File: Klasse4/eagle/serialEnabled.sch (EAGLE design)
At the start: 3 parts

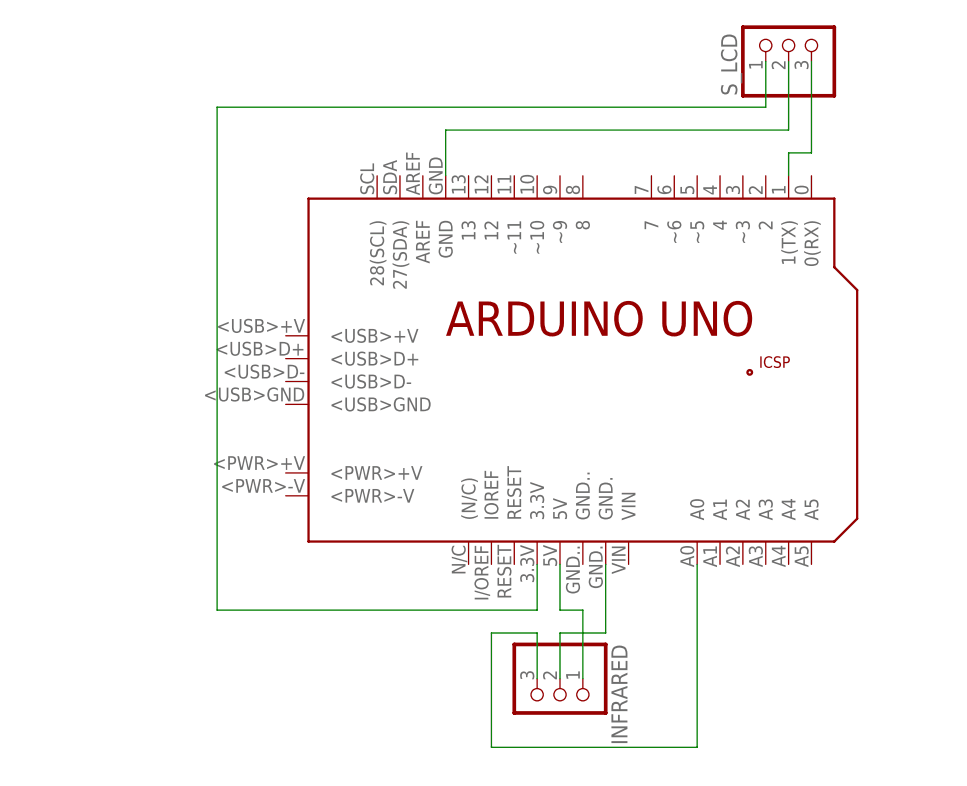
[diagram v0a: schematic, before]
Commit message: update
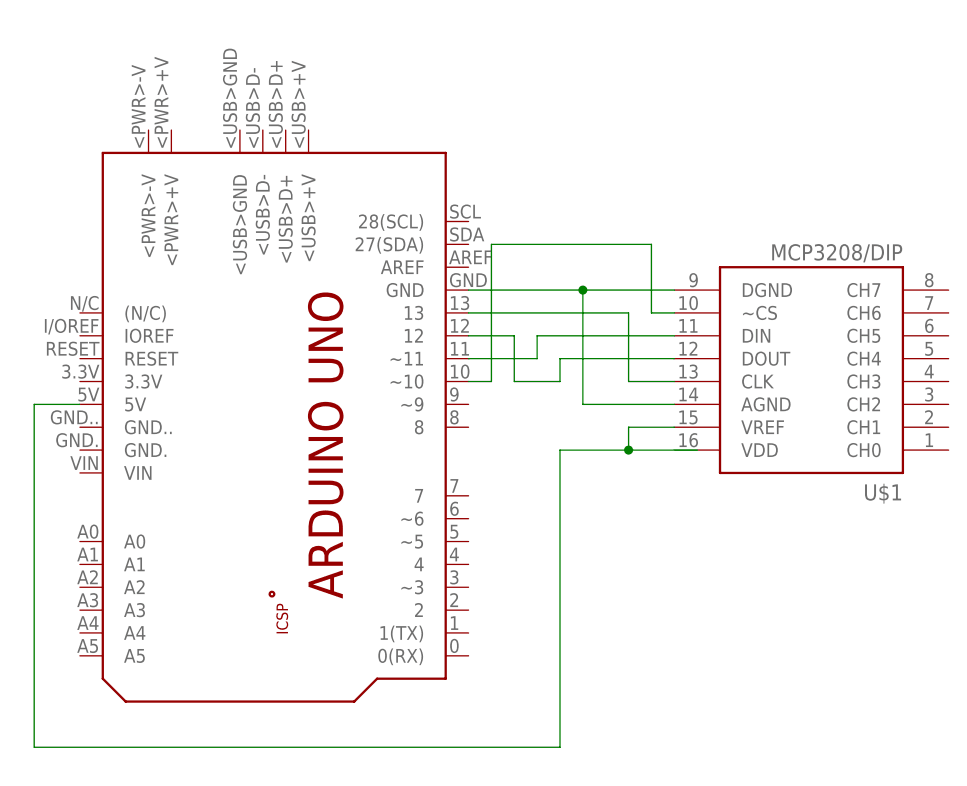
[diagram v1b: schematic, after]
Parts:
- removed INFRARED, S_LCD: (no value), pinhead:PINHD-1X3
- added U$1: MCP3208/DIP, mcp3208:MCP3208/DIP
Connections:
- net N$1: now also PCB1.GND, U$1.AGND, U$1.DGND; no longer INFRARED.1, PCB1.5V
- net N$2: now also PCB1.~11, U$1.DIN; no longer INFRARED.2, PCB1.GND.
- net N$3: now also PCB1.5V, U$1.VREF; no longer INFRARED.3, PCB1.A0
- net N$4: now also PCB1.13, U$1.CLK; no longer PCB1.1(TX), S_LCD.3
- net N$5: now also PCB1.12, U$1.DOUT; no longer PCB1.GND, S_LCD.2
- net N$6: now also PCB1.~10, U$1.~CS; no longer PCB1.3.3V, S_LCD.1
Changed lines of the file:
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@@
 <layer number="106" name="bPlate" color="7" fill="1" visible="yes" active="yes"/>
 <layer number="107" name="Crop" color="7" fill="1" visible="yes" active="yes"/>
+<layer number="108" name="fp8" color="7" fill="1" visible="no" active="yes"/>
+<layer number="109" name="fp9" color="7" fill="1" visible="no" active="yes"/>
+<layer number="110" name="fp0" color="7" fill="1" visible="no" active="yes"/>
+<layer number="111" name="LPC17xx" color="7" fill="1" visible="yes" active="yes"/>
 <layer number="116" name="Patch_BOT" color="9" fill="4" visible="yes" active="yes"/>
 <layer number="121" name="_tsilk" color="7" fill="1" visible="yes" active="yes"/>
 <layer number="122" name="_bsilk" color="7" fill="1" visible="yes" active="yes"/>
+<layer number="123" name="tTestmark" color="7" fill="1" visible="no" active="yes"/>
+<layer number="124" name="bTestmark" color="7" fill="1" visible="no" active="yes"/>
 <layer number="125" name="_tNames" color="7" fill="1" visible="yes" active="yes"/>
+<layer number="131" name="tAdjust" color="7" fill="1" visible="no" active="yes"/>
+<layer number="132" name="bAdjust" color="7" fill="1" visible="no" active="yes"/>
 <layer number="144" name="Drill_legend" color="7" fill="1" visible="yes" active="yes"/>
 <layer number="151" name="HeatSink" color="7" fill="1" visible="yes" active="yes"/>
+<layer number="199" name="Contour" color="7" fill="1" visible="yes" active="yes"/>
 <layer number="200" name="200bmp" color="1" fill="10" visible="yes" active="yes"/>
 <layer number="201" name="201bmp" color="2" fill="10" visible="yes" active="yes"/>
@@
 <parts>
 <part name="PCB1" library="E14_Arduino" deviceset="ARDUINO_UNO" device=""/>
-<part name="INFRARED" library="pinhead" deviceset="PINHD-1X3" device=""/>
-<part name="S_LCD" library="pinhead" deviceset="PINHD-1X3" device=""/>
+<part name="U$1" library="mcp3208" deviceset="MCP3208/DIP" device=""/>
 </parts>
 <sheets>
@@
 </plain>
 <instances>
-<instance part="PCB1" gate="G$1" x="2.54" y="30.48"/>
-<instance part="INFRARED" gate="A" x="0" y="-7.62" rot="R270"/>
-<instance part="S_LCD" gate="A" x="25.4" y="66.04" rot="R90"/>
+<instance part="PCB1" gate="G$1" x="-30.48" y="22.86" rot="R270"/>
+<instance part="U$1" gate="G$1" x="27.94" y="30.48" rot="R180"/>
 </instances>
 <busses>
@@
 <net name="N$1" class="0">
 <segment>
+<pinref part="PCB1" gate="G$1" pin="GND"/>
+<pinref part="U$1" gate="G$1" pin="DGND"/>
+<wire x1="-10.16" y1="38.1" x2="2.54" y2="38.1" width="0.1524" layer="91"/>
+<pinref part="U$1" gate="G$1" pin="AGND"/>
+<wire x1="2.54" y1="38.1" x2="12.7" y2="38.1" width="0.1524" layer="91"/>
+<wire x1="12.7" y1="25.4" x2="2.54" y2="25.4" width="0.1524" layer="91"/>
+<wire x1="2.54" y1="25.4" x2="2.54" y2="38.1" width="0.1524" layer="91"/>
+<junction x="2.54" y="38.1"/>
+</segment>
+</net>
+<net name="N$3" class="0">
+<segment>
 <pinref part="PCB1" gate="G$1" pin="5V"/>
-<wire x1="0" y1="7.62" x2="0" y2="2.54" width="0.1524" layer="91"/>
-<wire x1="0" y1="2.54" x2="2.54" y2="2.54" width="0.1524" layer="91"/>
-<pinref part="INFRARED" gate="A" pin="1"/>
-<wire x1="2.54" y1="2.54" x2="2.54" y2="-5.08" width="0.1524" layer="91"/>
+<wire x1="-53.34" y1="25.4" x2="-58.42" y2="25.4" width="0.1524" layer="91"/>
+<wire x1="-58.42" y1="25.4" x2="-58.42" y2="-12.7" width="0.1524" layer="91"/>
+<wire x1="-58.42" y1="-12.7" x2="0" y2="-12.7" width="0.1524" layer="91"/>
+<wire x1="0" y1="-12.7" x2="0" y2="20.32" width="0.1524" layer="91"/>
+<wire x1="0" y1="20.32" x2="7.62" y2="20.32" width="0.1524" layer="91"/>
+<pinref part="U$1" gate="G$1" pin="VREF"/>
+<wire x1="7.62" y1="20.32" x2="15.24" y2="20.32" width="0.1524" layer="91"/>
+<wire x1="12.7" y1="22.86" x2="7.62" y2="22.86" width="0.1524" layer="91"/>
+<wire x1="7.62" y1="22.86" x2="7.62" y2="20.32" width="0.1524" layer="91"/>
+<junction x="7.62" y="20.32"/>
 </segment>
 </net>
 <net name="N$2" class="0">
 <segment>
-<pinref part="PCB1" gate="G$1" pin="GND."/>
-<wire x1="5.08" y1="7.62" x2="5.08" y2="0" width="0.1524" layer="91"/>
-<wire x1="5.08" y1="0" x2="0" y2="0" width="0.1524" layer="91"/>
-<pinref part="INFRARED" gate="A" pin="2"/>
-<wire x1="0" y1="0" x2="0" y2="-5.08" width="0.1524" layer="91"/>
-</segment>
-</net>
-<net name="N$3" class="0">
-<segment>
-<pinref part="INFRARED" gate="A" pin="3"/>
-<wire x1="-2.54" y1="-5.08" x2="-2.54" y2="0" width="0.1524" layer="91"/>
-<wire x1="-2.54" y1="0" x2="-7.62" y2="0" width="0.1524" layer="91"/>
-<wire x1="-7.62" y1="0" x2="-7.62" y2="-12.7" width="0.1524" layer="91"/>
-<pinref part="PCB1" gate="G$1" pin="A0"/>
-<wire x1="-7.62" y1="-12.7" x2="15.24" y2="-12.7" width="0.1524" layer="91"/>
-<wire x1="15.24" y1="-12.7" x2="15.24" y2="7.62" width="0.1524" layer="91"/>
+<pinref part="PCB1" gate="G$1" pin="~11"/>
+<wire x1="-10.16" y1="30.48" x2="-2.54" y2="30.48" width="0.1524" layer="91"/>
+<wire x1="-2.54" y1="30.48" x2="-2.54" y2="33.02" width="0.1524" layer="91"/>
+<pinref part="U$1" gate="G$1" pin="DIN"/>
+<wire x1="12.7" y1="33.02" x2="-2.54" y2="33.02" width="0.1524" layer="91"/>
 </segment>
 </net>
 <net name="N$4" class="0">
 <segment>
-<pinref part="S_LCD" gate="A" pin="3"/>
-<wire x1="27.94" y1="63.5" x2="27.94" y2="53.34" width="0.1524" layer="91"/>
-<wire x1="27.94" y1="53.34" x2="25.4" y2="53.34" width="0.1524" layer="91"/>
-<pinref part="PCB1" gate="G$1" pin="1(TX)"/>
-<wire x1="25.4" y1="53.34" x2="25.4" y2="50.8" width="0.1524" layer="91"/>
+<pinref part="PCB1" gate="G$1" pin="13"/>
+<wire x1="-10.16" y1="35.56" x2="7.62" y2="35.56" width="0.1524" layer="91"/>
+<wire x1="7.62" y1="35.56" x2="7.62" y2="27.94" width="0.1524" layer="91"/>
+<pinref part="U$1" gate="G$1" pin="CLK"/>
+<wire x1="7.62" y1="27.94" x2="12.7" y2="27.94" width="0.1524" layer="91"/>
 </segment>
 </net>
 <net name="N$5" class="0">
 <segment>
-<pinref part="S_LCD" gate="A" pin="2"/>
-<wire x1="25.4" y1="63.5" x2="25.4" y2="55.88" width="0.1524" layer="91"/>
-<wire x1="25.4" y1="55.88" x2="-12.7" y2="55.88" width="0.1524" layer="91"/>
-<pinref part="PCB1" gate="G$1" pin="GND"/>
-<wire x1="-12.7" y1="55.88" x2="-12.7" y2="50.8" width="0.1524" layer="91"/>
+<pinref part="PCB1" gate="G$1" pin="12"/>
+<wire x1="-10.16" y1="33.02" x2="-5.08" y2="33.02" width="0.1524" layer="91"/>
+<wire x1="-5.08" y1="33.02" x2="-5.08" y2="27.94" width="0.1524" layer="91"/>
+<wire x1="-5.08" y1="27.94" x2="0" y2="27.94" width="0.1524" layer="91"/>
+<wire x1="0" y1="27.94" x2="0" y2="30.48" width="0.1524" layer="91"/>
+<pinref part="U$1" gate="G$1" pin="DOUT"/>
+<wire x1="0" y1="30.48" x2="12.7" y2="30.48" width="0.1524" layer="91"/>
 </segment>
 </net>
 <net name="N$6" class="0">
 <segment>
-<pinref part="S_LCD" gate="A" pin="1"/>
-<wire x1="22.86" y1="63.5" x2="22.86" y2="58.42" width="0.1524" layer="91"/>
-<wire x1="22.86" y1="58.42" x2="-38.1" y2="58.42" width="0.1524" layer="91"/>
-<wire x1="-38.1" y1="58.42" x2="-38.1" y2="2.54" width="0.1524" layer="91"/>
-<pinref part="PCB1" gate="G$1" pin="3.3V"/>
-<wire x1="-38.1" y1="2.54" x2="-2.54" y2="2.54" width="0.1524" layer="91"/>
-<wire x1="-2.54" y1="2.54" x2="-2.54" y2="7.62" width="0.1524" layer="91"/>
+<pinref part="PCB1" gate="G$1" pin="~10"/>
+<wire x1="-10.16" y1="27.94" x2="-7.62" y2="27.94" width="0.1524" layer="91"/>
+<wire x1="-7.62" y1="27.94" x2="-7.62" y2="43.18" width="0.1524" layer="91"/>
+<wire x1="-7.62" y1="43.18" x2="10.16" y2="43.18" width="0.1524" layer="91"/>
+<wire x1="10.16" y1="43.18" x2="10.16" y2="35.56" width="0.1524" layer="91"/>
+<pinref part="U$1" gate="G$1" pin="~CS"/>
+<wire x1="10.16" y1="35.56" x2="12.7" y2="35.56" width="0.1524" layer="91"/>
 </segment>
 </net>
